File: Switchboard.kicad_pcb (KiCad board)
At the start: 2 copper layers, 54.6 x 48.9 mm, 22 parts, among them J2 Conn_01x02_Female, J3 AudioJack2_SwitchT, J4 Conn_01x06_Female, J5 AudioJack2_SwitchT, SW1 SW_3PDT_x3, U101 LTC1044

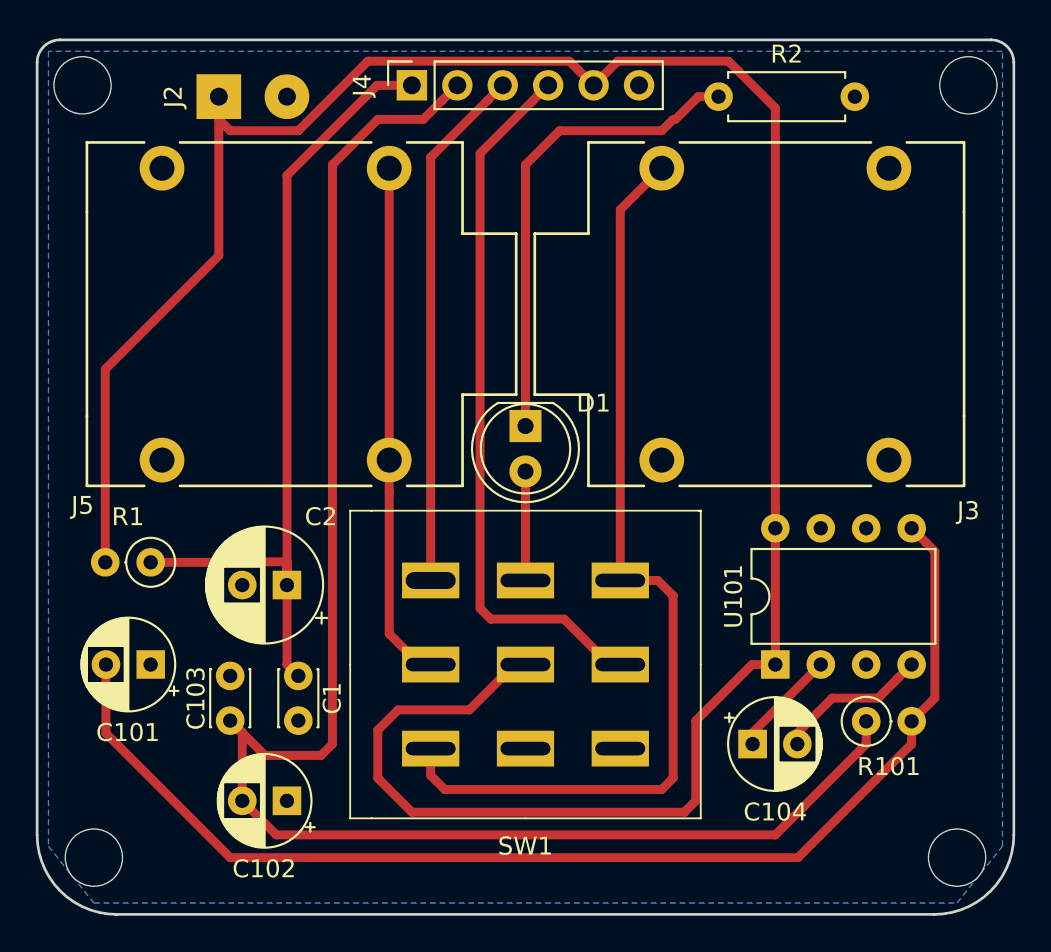
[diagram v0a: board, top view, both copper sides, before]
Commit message: Migrate to KiCAD 6!
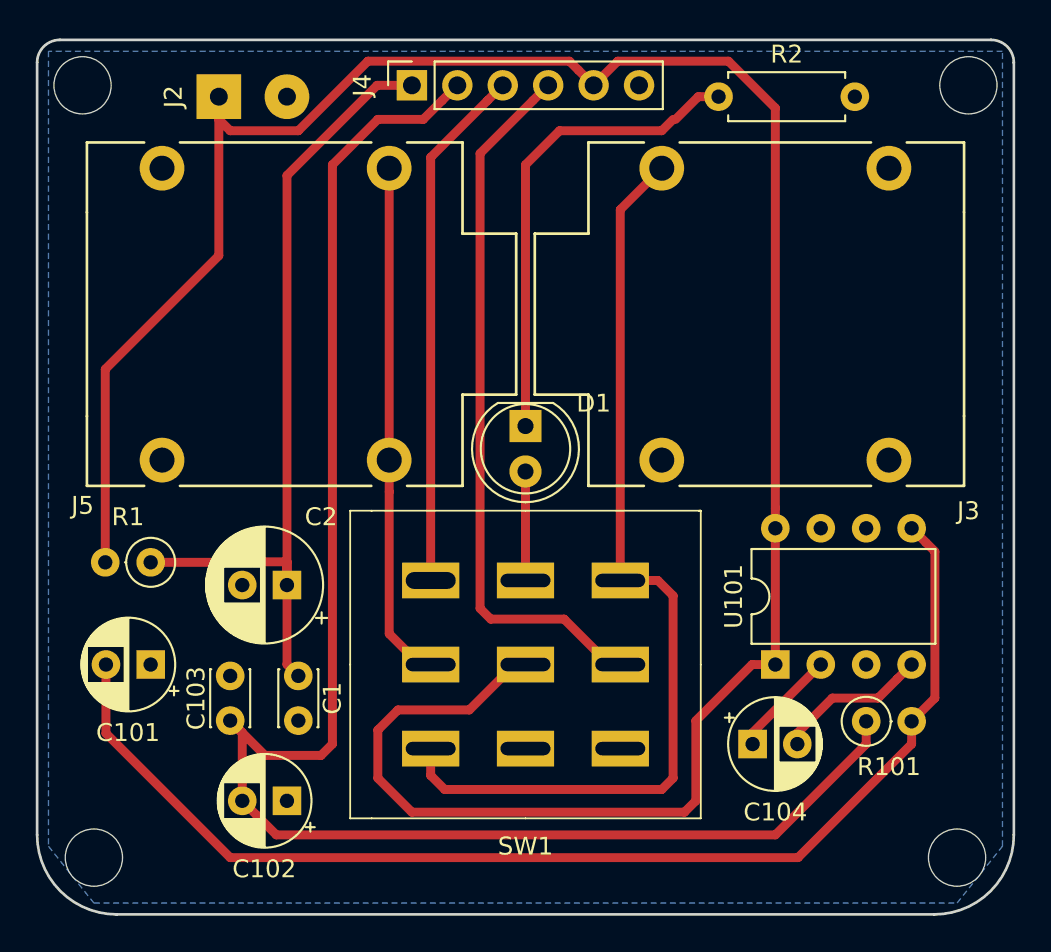
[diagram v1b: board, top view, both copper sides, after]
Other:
- net class Default removed
